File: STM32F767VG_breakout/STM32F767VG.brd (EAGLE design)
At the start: 89.8 x 43.8 mm, 42 parts, among them IC1 STM32F767VGT6, IC2 L7805CV, IC3 LD117AS33TR, X4 8MHz, X5 32.768kHz

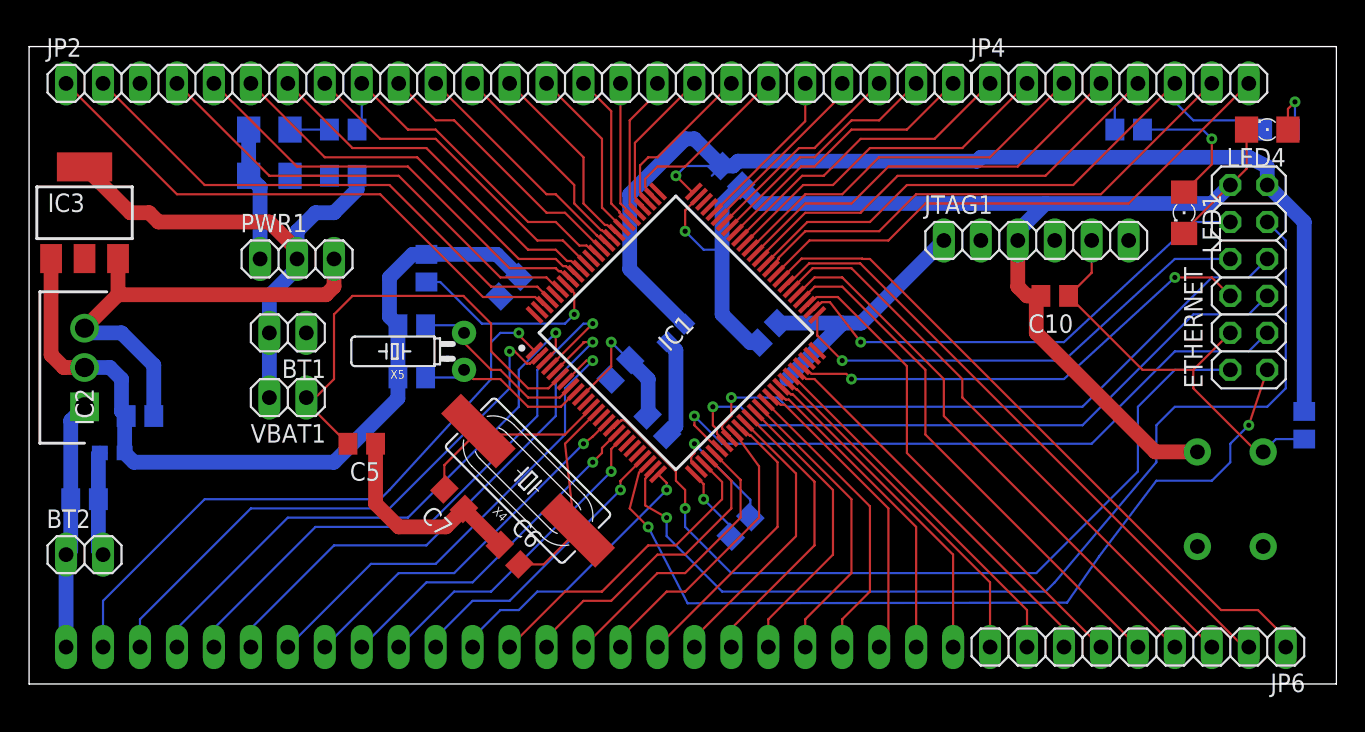
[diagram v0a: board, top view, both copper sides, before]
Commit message: First complete routing
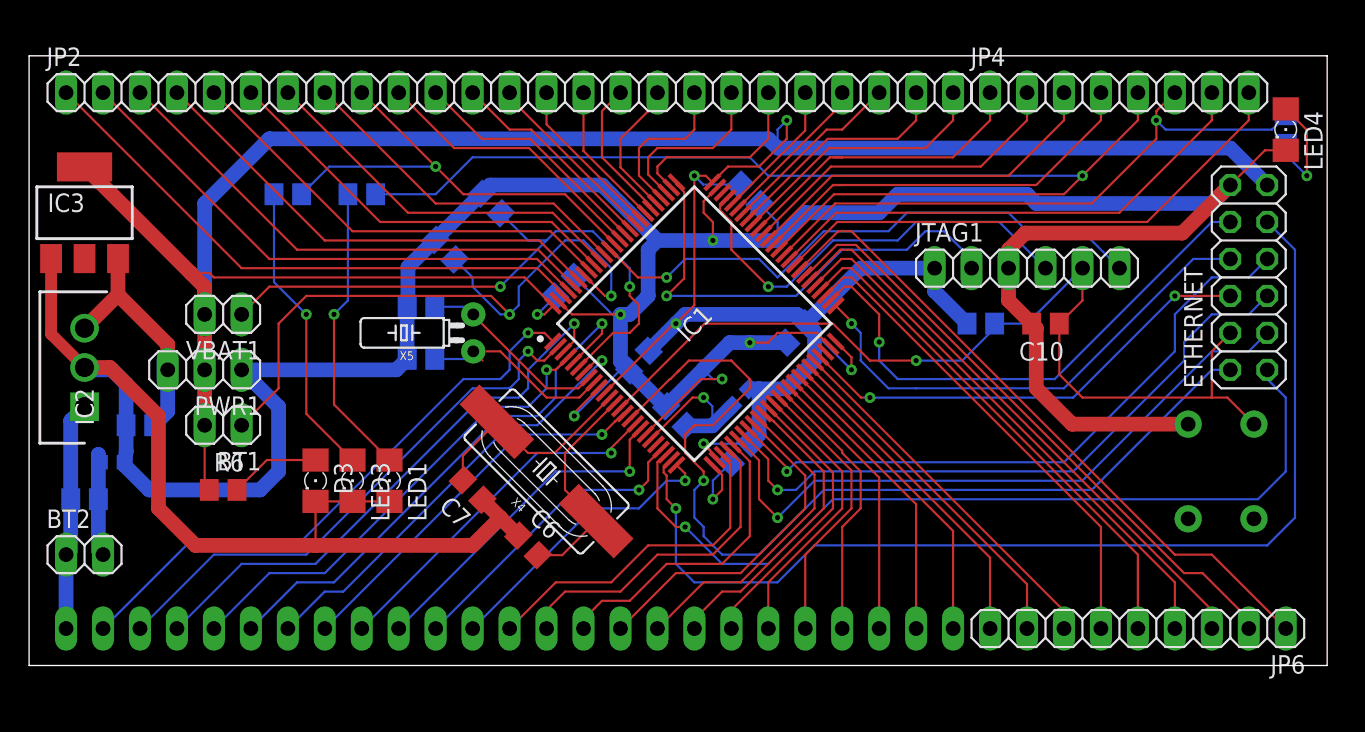
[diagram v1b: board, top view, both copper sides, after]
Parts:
- moved LED1 57.6 mm to (24.8, 29.2)
- moved R3 52.9 mm to (22.9, 48.9), turned to 0 degrees
- moved LED3 24.8 mm to (22.2, 29.2), flipped to the top, turned to 270 degrees
- moved R1 23.3 mm to (65.4, 40.0), turned to 180 degrees
- moved R6 23.1 mm to (13.3, 28.6), flipped to the top
- moved D3 21.2 mm to (19.7, 29.2), flipped to the top, turned to 270 degrees
- moved C5 18.8 mm to (31.8, 48.3), flipped to the bottom, turned to 225 degrees
- moved PWR1 9.92 mm to (12.1, 36.8), turned to 180 degrees
- moved BT1 7.75 mm to (13.3, 33.0)
- moved VBAT1 7.24 mm to (13.3, 40.6)
- moved BEAD3 6.29 mm to (48.9, 34.9)
- moved R7 5.85 mm to (17.8, 48.9)
- moved C13 5.08 mm to (48.9, 31.1)
- moved C11 3.81 mm to (36.8, 42.5)
- moved JTAG1 2.01 mm to (68.6, 43.8)
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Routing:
- net GND: track 185.1 -> 280.7 mm, vias 3 -> 6
- net VDD: track 144.9 -> 221.7 mm, vias 2 -> 6
- net PD15: track 34.8 -> 80.4 mm, vias 0 -> 1
- net SWO: track 0.00 -> 40.3 mm, vias 0 -> 1
- net NRST: track 29.8 -> 65.9 mm, vias 0 -> 1
- net PB9: track 0.00 -> 35.3 mm
- net TCK: track 0.00 -> 32.7 mm, vias 0 -> 1
- net BOOT0: track 13.9 -> 45.9 mm, vias 1 -> 2
- net TMS: track 0.00 -> 30.1 mm, vias 0 -> 1
- net N$26: track 2.71 -> 20.5 mm, vias 0 -> 1
- net 5V: track 32.0 -> 16.5 mm
- net N$13: track 31.4 -> 43.5 mm, vias 0 -> 2
- net N$17: track 9.48 -> 20.2 mm
- net MDC: track 57.3 -> 67.1 mm
- net PE5: track 42.0 -> 32.8 mm
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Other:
- board size 89.8 x 43.8 mm -> 89.2 x 41.9 mm
